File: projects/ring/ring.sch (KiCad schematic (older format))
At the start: 35 parts, among them U1 STM32WB55CEU6TR, U2 LSM6DSO32TR, U3 ANT016008LCS2442MA2, U4 BQ297xy, U5 TPS62840DLCR, Y1 NX1612SA-32.000MHZ-CHP-CIS-3

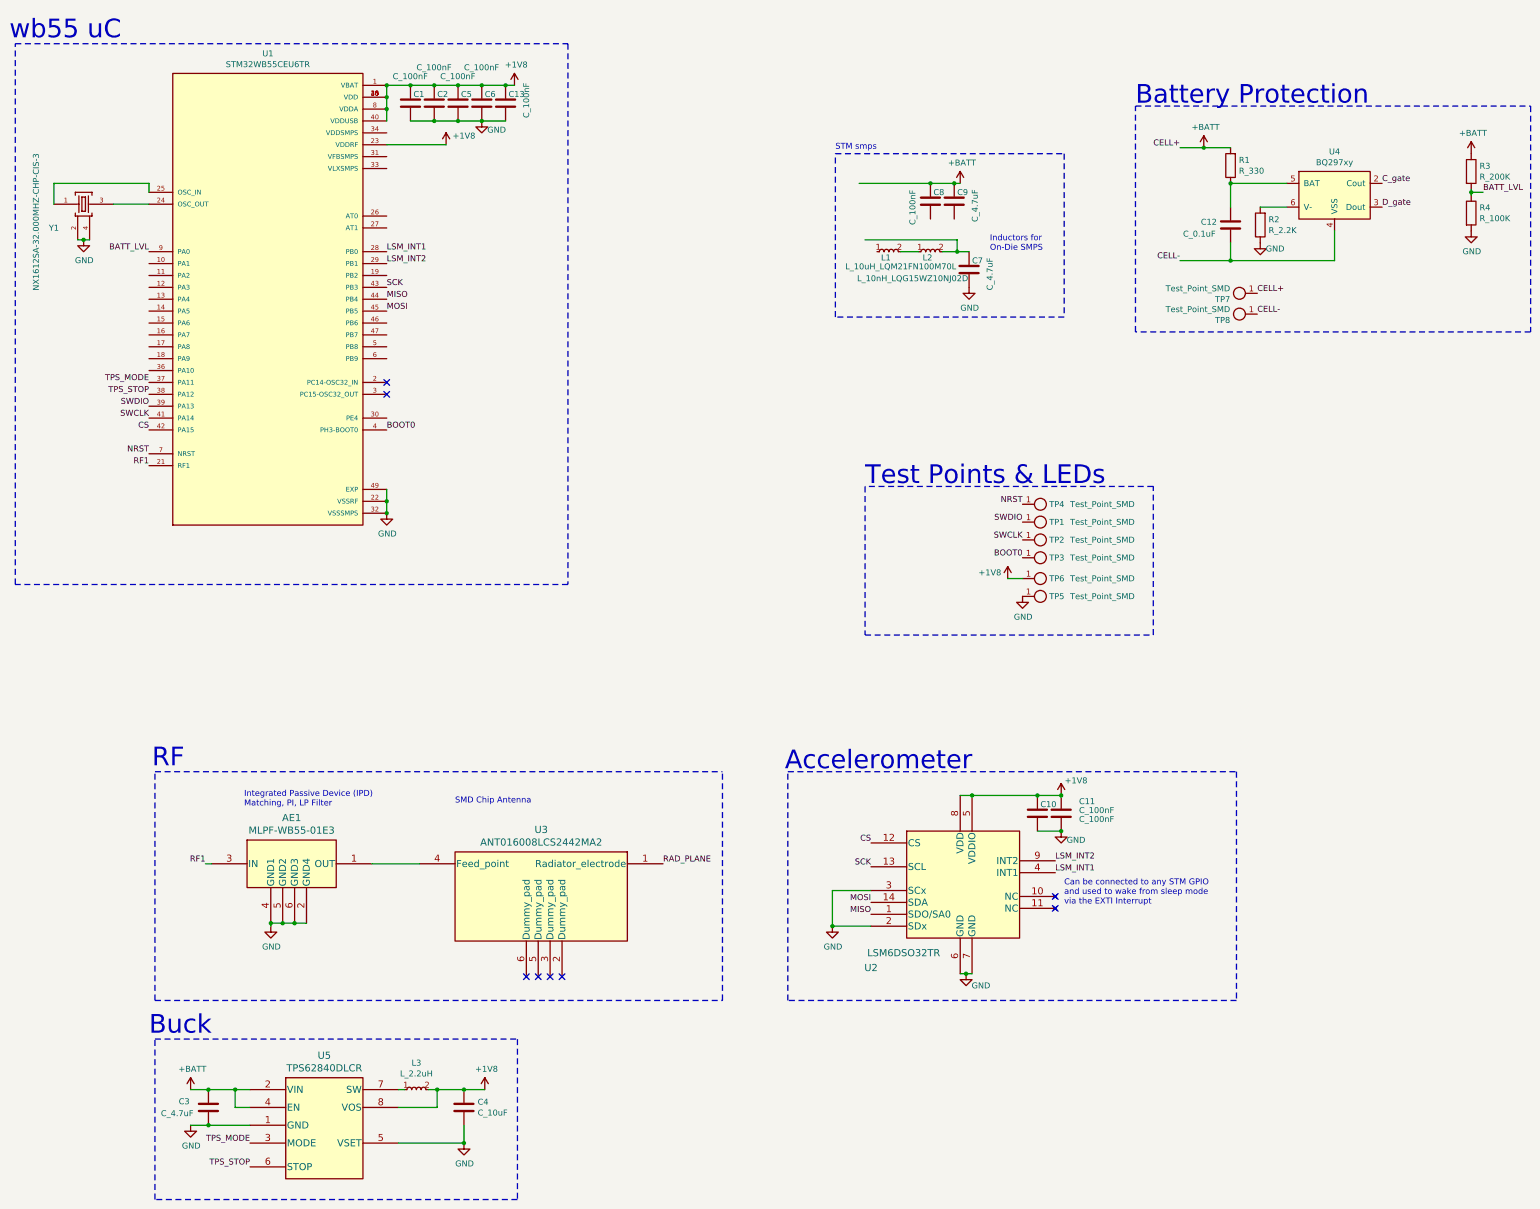
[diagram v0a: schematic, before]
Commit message: an inch closer to hardware first rev completion
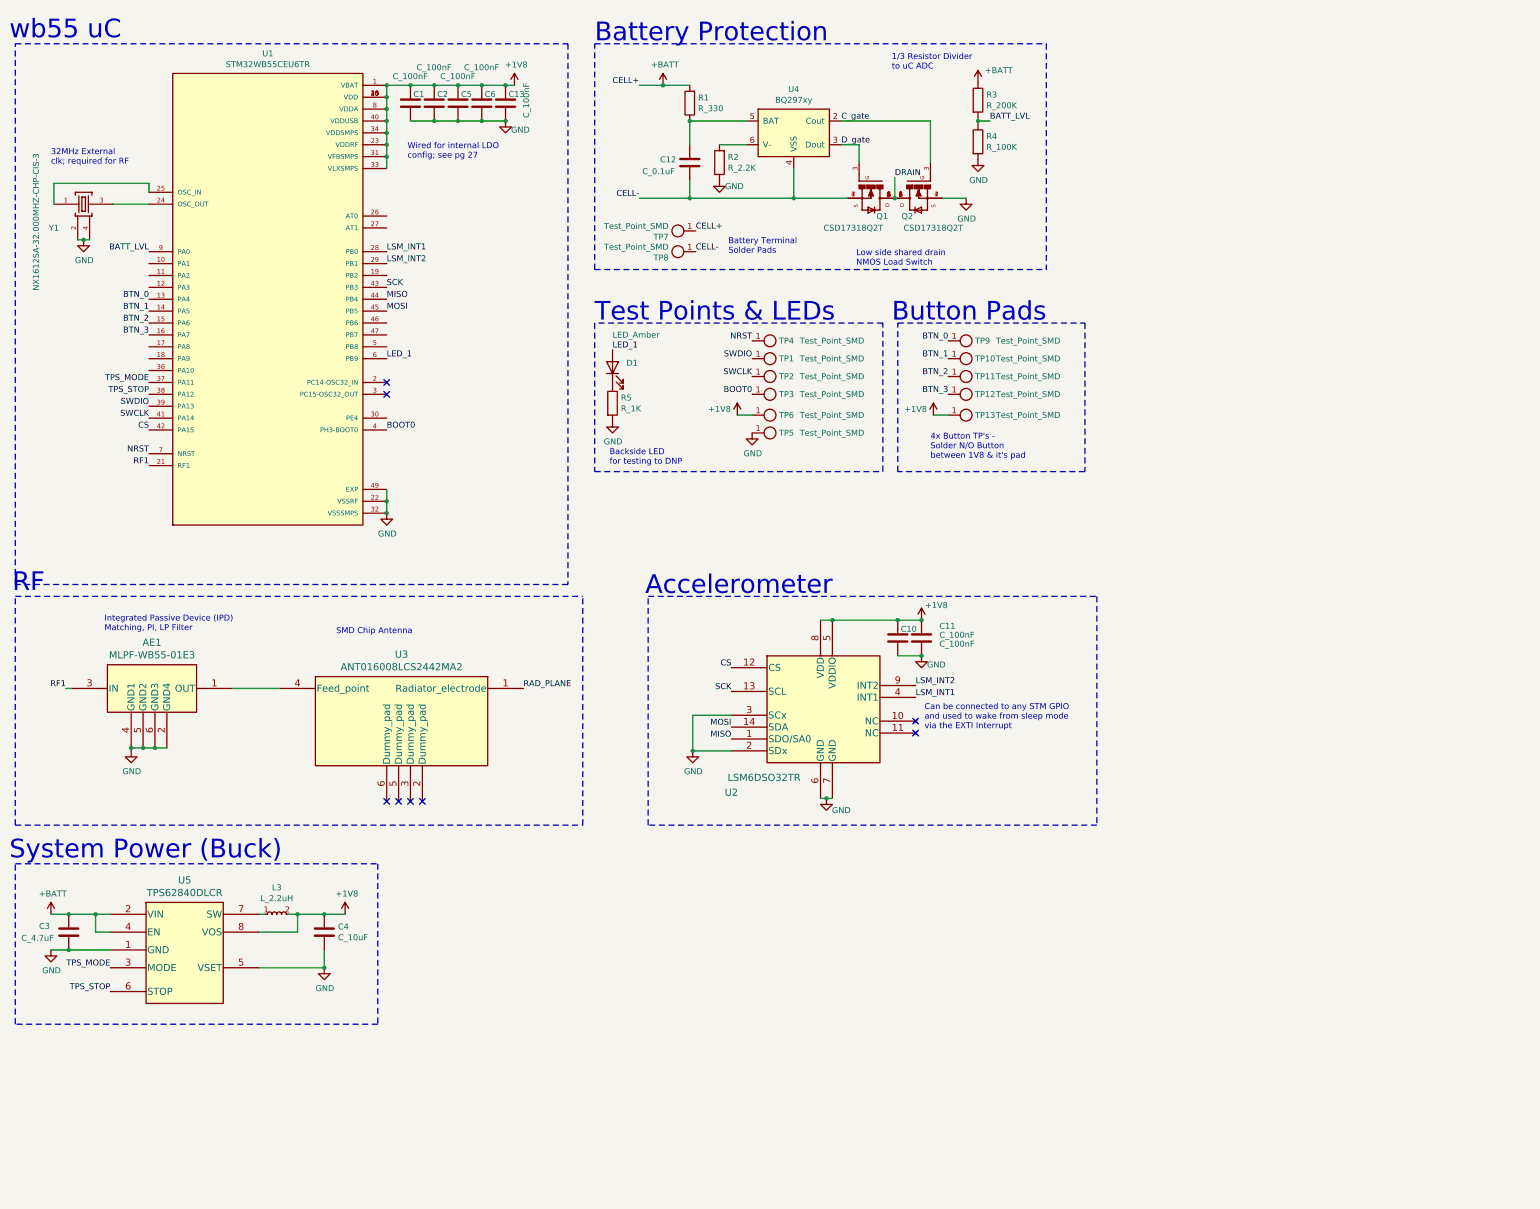
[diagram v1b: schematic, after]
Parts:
- removed C7, C9: C_4.7uF, Capacitor_SMD:C_0402_1005Metric, symbol step:C_4.7uF
- removed C8: C_100nF, Capacitor_SMD:C_0402_1005Metric, symbol step:C_100nF
- removed L1: L_10uH_LQM21FN100M70L, Inductor_SMD:L_0805_2012Metric, symbol step:L_10uH_LQM21FN100M70L
- removed L2: L_10nH_LQG15WZ10NJ02D, Inductor_SMD:L_0402_1005Metric, symbol step:L_10nH_LQG15WZ10NJ02D
- added D1: LED_Amber, LED_SMD:LED_0402_1005Metric, symbol step:LED_0805_Amber
- added Q1, Q2: CSD17318Q2T, step-footprints:TRANS_CSD17318Q2T, symbol step:CSD17318Q2T
- added R5: R_1K, Resistor_SMD:R_0402_1005Metric, symbol step:R_1K
- added TP10, TP11, TP12, TP13, TP9: Test_Point_SMD, TestPoint:TestPoint_Pad_1.0x1.0mm, symbol step:Test_Point_SMD
- AE1: buy (none) -> https://www.digikey.com/en/products/detail/stmicroelectroni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
- TP7, TP8: footprint TestPoint:TestPoint_Pad_2.0x2.0mm -> TestPoint:TestPoint_Pad_1.5x1.5mm
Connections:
- net +1V8: now also U1.31 (VFBSMPS), U1.33 (VLXSMPS), U1.34 (VDDSMPS), TP13.1
- net CELL-: now also Q1.4, Q1.7
- net C_gate: now also Q2.3
- net D_gate: now also Q1.3
- net GND: now also Q2.4, Q2.7, R5.2
- net BTN_0: now reaches U1.13 (PA4)
- net BTN_0: now also TP9.1
- net BTN_1: now reaches U1.14 (PA5)
- net BTN_1: now also TP10.1
- net BTN_2: now reaches U1.15 (PA6)
- net BTN_2: now also TP11.1
- net BTN_3: now reaches U1.16 (PA7)
- net BTN_3: now also TP12.1
- net LED_1: now reaches U1.6 (PB9)
- net LED_1: now also D1.2 (A)
- new net: D1.1 (K), R5.1
- new net DRAIN: Q1.1, Q1.2, Q1.5, Q1.6, Q1.8, Q2.1, Q2.2, Q2.5, Q2.6, Q2.8
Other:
- note added: "1/3 Resistor Divider \nto uC ADC"
- note added: "32MHz External \nclk; required for RF"
- note added: "4x Button TP's - \nSolder N/O Button \nbetween 1V8 & it's pad"
- note added: "Backside LED\nfor testing to DNP"
- note added: "Battery Terminal\nSolder Pads\n"
- note added: "Button Pads"
- note added: "Low side shared drain \nNMOS Load Switch \n"
- note added: "System Power (Buck)"
- note added: "Wired for internal LDO \nconfig; see pg 27"
- note removed: "Buck"
- note removed: "Inductors for \nOn-Die SMPS"
- note removed: "STM smps"
- moved on the sheet: AE1, C10, C11, C12, C3, C4, L3, R1, R2, R3, R4, TP1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
